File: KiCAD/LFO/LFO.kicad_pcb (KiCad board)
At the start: 2 copper layers, 30 x 100 mm, 16 parts, among them J1 OUT, J2 OUT, J3 Conn_01x03, J4 Conn_01x03, SW1 SW_SPDT, U1 TL072

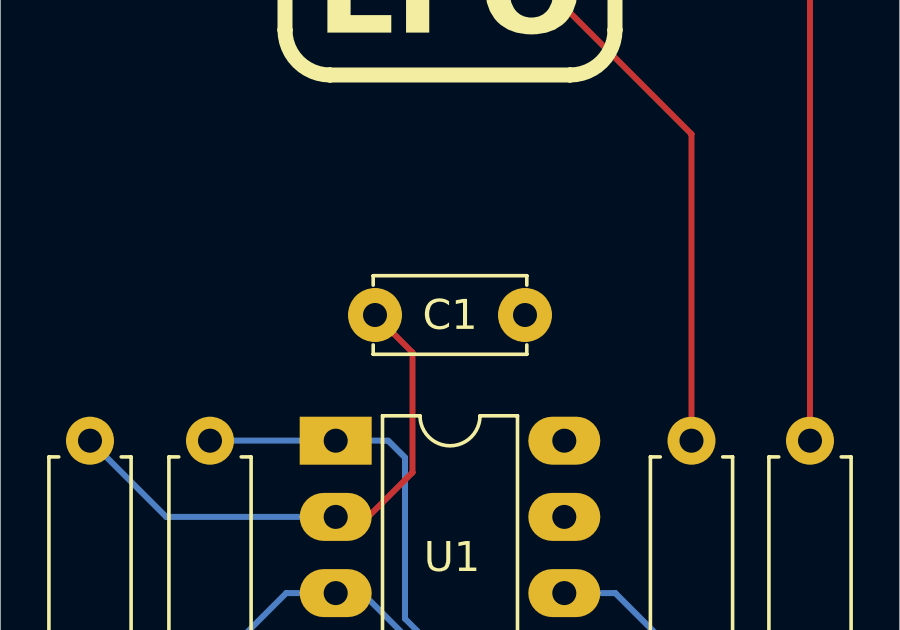
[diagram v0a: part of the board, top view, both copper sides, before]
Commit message: Library updates
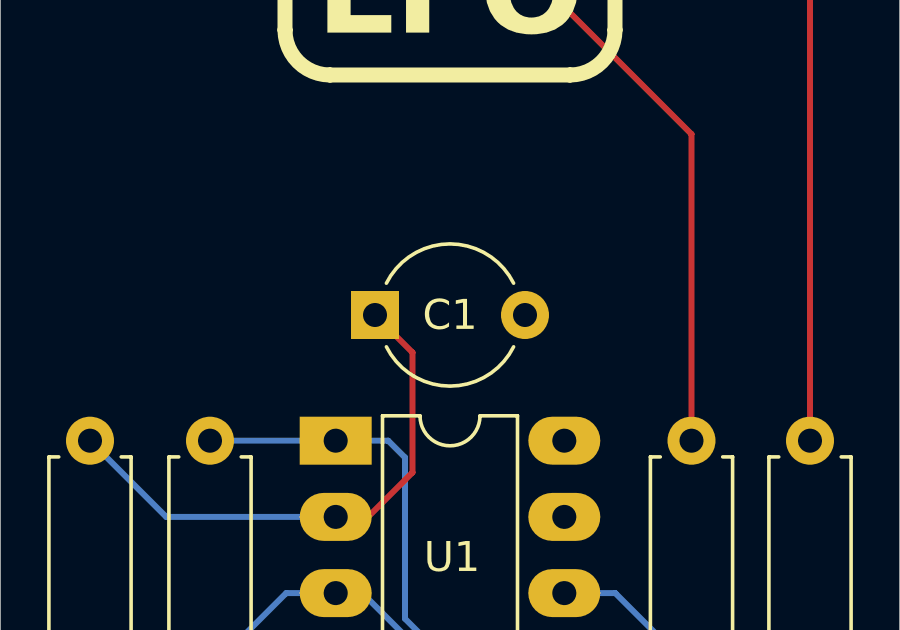
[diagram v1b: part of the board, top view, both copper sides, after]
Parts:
- C1: footprint HackSynth:C_Disc_D5.0mm_W2.5mm_P5.00mm -> HackSynth:C_Radial_Tantal_D4.5mm_P5.00mm
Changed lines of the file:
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@@
 		)
 		(embedded_fonts no)
-		(model "C:/Program Files/KiCad/share/kicad/modules/packages3d/Package_DIP.3dshapes/DIP-8_W7.62mm.step"
+		(model "C:/Users/ocd/OneDrive/Drafting/CCHS/HackSynth/KiCAD/HackSynth.pretty/DIP-8_W7.62mm.step"
 			(offset
 				(xyz -3.81 3.81 0)
@@
 		)
 	)
-	(footprint "HackSynth:C_Disc_D5.0mm_W2.5mm_P5.00mm"
+	(footprint "HackSynth:C_Radial_Tantal_D4.5mm_P5.00mm"
 		(layer "F.Cu")
 		(at 147.5 92)
-		(descr "C, Disc series, Radial, pin pitch=5.00mm, , diameter*width=5*2.5mm^2, Capacitor, http://cdn-reichelt.de/documents/datenblatt/B300/DS_KERKO_TC.pdf")
-		(tags "C Disc series Radial pin pitch 5.00mm  diameter 5mm width 2.5mm Capacitor")
+		(descr "CP, Radial_Tantal series, Radial, pin pitch=5.00mm, diameter=4.5mm, height=10mm, Tantal Electrolytic Capacitor, http://cdn-reichelt.de/documents/datenblatt/B300/TANTAL-TB-Serie%23.pdf")
+		(tags "CP Radial_Tantal series Radial pin pitch 5.00mm diameter 4.5mm height 10mm Tantal Electrolytic Capacitor")
 		(property "Reference" "C1"
 			(at 2.5 0 0)
@@
 		)
 		(property "Value" "2µ2"
-			(at 2.5 -3 0)
+			(at 2.5 3.5 0)
 			(layer "F.Fab")
 			(effects
@@
 		(sheetfile "LFO.kicad_sch")
 		(attr through_hole)
-		(fp_line
-			(start -0.06 -1.31)
-			(end -0.06 -0.996)
+		(fp_arc
+			(start 0.380259 -1.06)
+			(mid 2.5 -2.37)
+			(end 4.619741 -1.06)
 			(stroke
 				(width 0.12)
@@
 			(layer "F.SilkS")
 		)
-		(fp_line
-			(start -0.06 -1.31)
-			(end 5.06 -1.31)
+		(fp_arc
+			(start 4.619741 1.06)
+			(mid 2.5 2.37)
+			(end 0.380259 1.06)
 			(stroke
 				(width 0.12)
@@
 			(layer "F.SilkS")
 		)
-		(fp_line
-			(start -0.06 0.996)
-			(end -0.06 1.31)
-			(stroke
-				(width 0.12)
-				(type solid)
-			)
-			(layer "F.SilkS")
-		)
-		(fp_line
-			(start -0.06 1.31)
-			(end 5.06 1.31)
-			(stroke
-				(width 0.12)
-				(type solid)
-			)
-			(layer "F.SilkS")
-		)
-		(fp_line
-			(start 5.06 -1.31)
-			(end 5.06 -0.996)
-			(stroke
-				(width 0.12)
-				(type solid)
-			)
-			(layer "F.SilkS")
-		)
-		(fp_line
-			(start 5.06 0.996)
-			(end 5.06 1.31)
-			(stroke
-				(width 0.12)
-				(type solid)
-			)
-			(layer "F.SilkS")
-		)
-		(fp_line
-			(start -1.05 -1.6)
-			(end -1.05 1.6)
+		(fp_circle
+			(center 2.5 0)
+			(end 6.22 0)
 			(stroke
 				(width 0.05)
 				(type solid)
 			)
+			(fill no)
 			(layer "F.CrtYd")
 		)
-		(fp_line
-			(start -1.05 1.6)
-			(end 6.05 1.6)
-			(stroke
-				(width 0.05)
-				(type solid)
-			)
-			(layer "F.CrtYd")
-		)
-		(fp_line
-			(start 6.05 -1.6)
-			(end -1.05 -1.6)
-			(stroke
-				(width 0.05)
-				(type solid)
-			)
-			(layer "F.CrtYd")
-		)
-		(fp_line
-			(start 6.05 1.6)
-			(end 6.05 -1.6)
-			(stroke
-				(width 0.05)
-				(type solid)
-			)
-			(layer "F.CrtYd")
-		)
-		(fp_line
-			(start 0 -1.25)
-			(end 0 1.25)
+		(fp_circle
+			(center 2.5 0)
+			(end 4.75 0)
 			(stroke
 				(width 0.1)
 				(type solid)
 			)
-			(layer "F.Fab")
-		)
-		(fp_line
-			(start 0 1.25)
-			(end 5 1.25)
-			(stroke
-				(width 0.1)
-				(type solid)
-			)
-			(layer "F.Fab")
-		)
-		(fp_line
-			(start 5 -1.25)
-			(end 0 -1.25)
-			(stroke
-				(width 0.1)
-				(type solid)
-			)
-			(layer "F.Fab")
-		)
-		(fp_line
-			(start 5 1.25)
-			(end 5 -1.25)
-			(stroke
-				(width 0.1)
-				(type solid)
-			)
+			(fill no)
 			(layer "F.Fab")
 		)
@@
 			(effects
 				(font
-					(size 1 1)
-					(thickness 0.15)
+					(size 0.9 0.9)
+					(thickness 0.135)
 				)
 			)
 		)
-		(pad "1" thru_hole circle
+		(pad "1" thru_hole rect
 			(at 0 0)
-			(size 1.8 1.8)
+			(size 1.6 1.6)
 			(drill 0.8)
 			(layers "*.Cu" "*.Mask")
@@
 		(pad "2" thru_hole circle
 			(at 5 0)
-			(size 1.8 1.8)
+			(size 1.6 1.6)
 			(drill 0.8)
 			(layers "*.Cu" "*.Mask")
@@
 		)
 		(embedded_fonts no)
-		(model "C:/Program Files/KiCad/share/kicad/modules/packages3d/Capacitor_THT.3dshapes/C_Disc_D5.0mm_W2.5mm_P5.00mm.step"
+		(model "${KICAD9_3DMODEL_DIR}/Capacitor_THT.3dshapes/CP_Radial_Tantal_D4.5mm_P5.00mm.wrl"
 			(offset
 				(xyz 0 0 0)

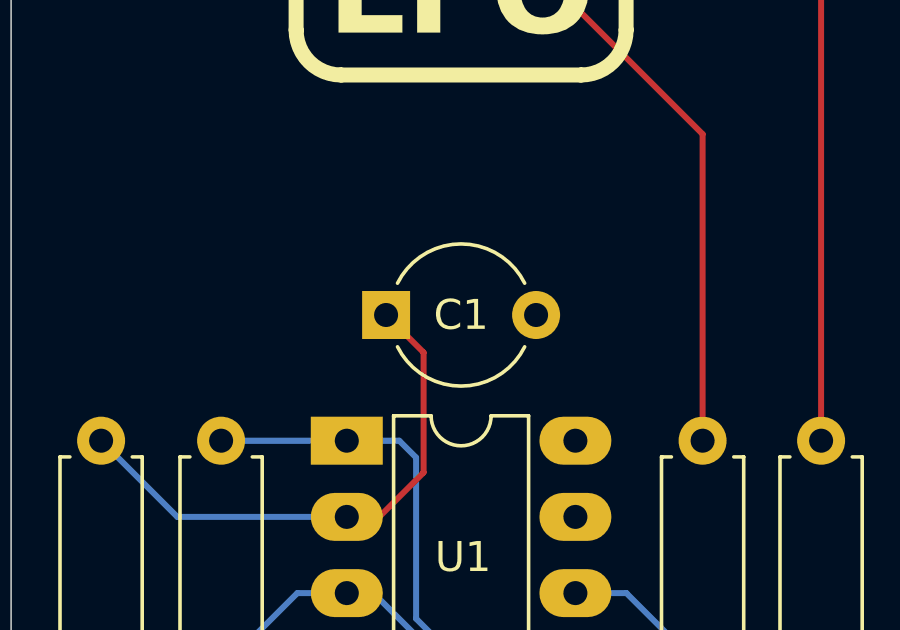
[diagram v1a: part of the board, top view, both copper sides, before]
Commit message: ASDR Schematic + LFO Gerbers
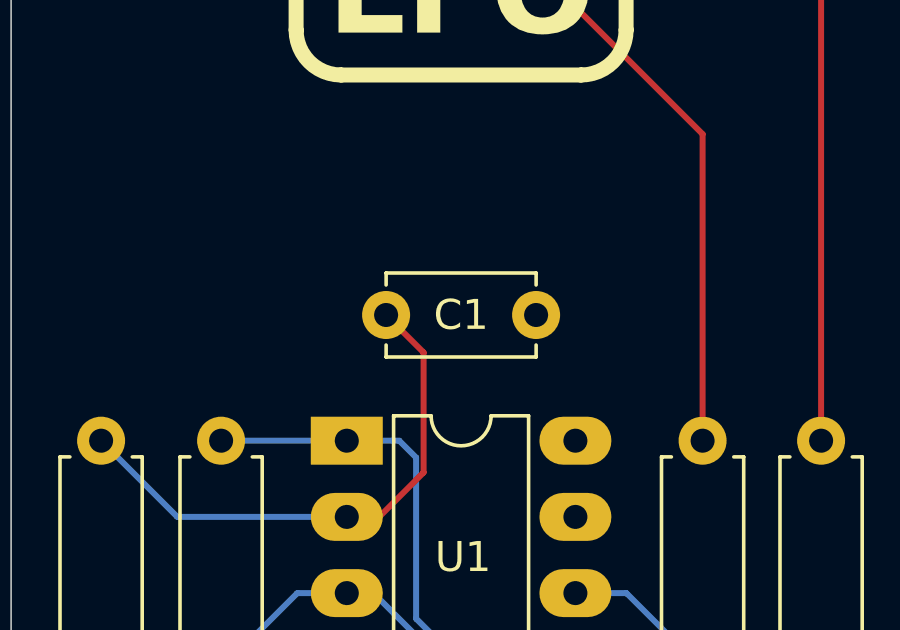
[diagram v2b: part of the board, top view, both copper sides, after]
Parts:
- C1: footprint HackSynth:C_Radial_Tantal_D4.5mm_P5.00mm -> HackSynth:C_Ceramic_D4.5mm_P5.00mm
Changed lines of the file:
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@@
 		(tenting front back)
 		(pcbplotparams
-			(layerselection 0x00000000_00000000_55555555_5755f5ff)
+			(layerselection 0x00000000_00000000_55555555_575555ff)
 			(plot_on_all_layers_selection 0x00000000_00000000_00000000_00000000)
 			(disableapertmacros no)
@@
 			(usegerberattributes yes)
 			(usegerberadvancedattributes yes)
-			(creategerberjobfile yes)
+			(creategerberjobfile no)
 			(dashed_line_dash_ratio 12.000000)
 			(dashed_line_gap_ratio 3.000000)
@@
 			(outputformat 1)
 			(mirror no)
-			(drillshape 1)
+			(drillshape 0)
 			(scaleselection 1)
-			(outputdirectory "")
+			(outputdirectory "Gerbers/")
 		)
 	)
@@
 		)
 	)
-	(footprint "HackSynth:C_Radial_Tantal_D4.5mm_P5.00mm"
+	(footprint "HackSynth:C_Ceramic_D4.5mm_P5.00mm"
 		(layer "F.Cu")
 		(at 147.5 92)
-		(descr "CP, Radial_Tantal series, Radial, pin pitch=5.00mm, diameter=4.5mm, height=10mm, Tantal Electrolytic Capacitor, http://cdn-reichelt.de/documents/datenblatt/B300/TANTAL-TB-Serie%23.pdf")
-		(tags "CP Radial_Tantal series Radial pin pitch 5.00mm diameter 4.5mm height 10mm Tantal Electrolytic Capacitor")
 		(property "Reference" "C1"
-			(at 2.5 0 0)
+			(at 2.5 0.000001 0)
 			(layer "F.SilkS")
 			(effects
@@
 		(sheetfile "LFO.kicad_sch")
 		(attr through_hole)
-		(fp_arc
-			(start 0.380259 -1.06)
-			(mid 2.5 -2.37)
-			(end 4.619741 -1.06)
+		(fp_line
+			(start 0 -1.4)
+			(end 5 -1.4)
 			(stroke
 				(width 0.12)
@@
 			(layer "F.SilkS")
 		)
-		(fp_arc
-			(start 4.619741 1.06)
-			(mid 2.5 2.37)
-			(end 0.380259 1.06)
+		(fp_line
+			(start 0 -1)
+			(end 0 -1.4)
 			(stroke
 				(width 0.12)
@@
 			(layer "F.SilkS")
 		)
-		(fp_circle
-			(center 2.5 0)
-			(end 6.22 0)
+		(fp_line
+			(start 0 1)
+			(end 0 1.4)
 			(stroke
-				(width 0.05)
+				(width 0.12)
 				(type solid)
 			)
+			(layer "F.SilkS")
+		)
+		(fp_line
+			(start 0 1.4)
+			(end 5 1.4)
+			(stroke
+				(width 0.12)
+				(type solid)
+			)
+			(layer "F.SilkS")
+		)
+		(fp_line
+			(start 5 -1.4)
+			(end 5 -1)
+			(stroke
+				(width 0.12)
+				(type solid)
+			)
+			(layer "F.SilkS")
+		)
+		(fp_line
+			(start 5 1.4)
+			(end 5 1)
+			(stroke
+				(width 0.12)
+				(type solid)
+			)
+			(layer "F.SilkS")
+		)
+		(fp_rect
+			(start -0.8 -1.5)
+			(end 5.8 1.5)
+			(stroke
+				(width 0.05)
+				(type default)
+			)
 			(fill no)
 			(layer "F.CrtYd")
 		)
-		(fp_circle
-			(center 2.5 0)
-			(end 4.75 0)
+		(fp_line
+			(start 0.1 -1.3)
+			(end 4.9 -1.3)
 			(stroke
 				(width 0.1)
-				(type solid)
+				(type default)
+			)
+			(layer "F.Fab")
+		)
+		(fp_line
+			(start 0.1 -0.9)
+			(end 0.1 -1.3)
+			(stroke
+				(width 0.1)
+				(type default)
+			)
+			(layer "F.Fab")
+		)
+		(fp_line
+			(start 0.1 0.9)
+			(end 0.1 1.3)
+			(stroke
+				(width 0.1)
+				(type default)
+			)
+			(layer "F.Fab")
+		)
+		(fp_line
+			(start 0.1 1.3)
+			(end 4.9 1.3)
+			(stroke
+				(width 0.1)
+				(type default)
+			)
+			(layer "F.Fab")
+		)
+		(fp_line
+			(start 4.9 -1.3)
+			(end 4.9 -0.9)
+			(stroke
+				(width 0.1)
+				(type default)
+			)
+			(layer "F.Fab")
+		)
+		(fp_line
+			(start 4.9 0.9)
+			(end 4.9 1.3)
+			(stroke
+				(width 0.1)
+				(type default)
 			)
-			(fill no)
 			(layer "F.Fab")
 		)
@@
 			)
 		)
-		(pad "1" thru_hole rect
+		(pad "1" thru_hole circle
 			(at 0 0)
 			(size 1.6 1.6)
@@
 		)
 		(embedded_fonts no)
-		(model "${KICAD9_3DMODEL_DIR}/Capacitor_THT.3dshapes/CP_Radial_Tantal_D4.5mm_P5.00mm.wrl"
+		(model "C:/Users/ocd/OneDrive/Drafting/CCHS/HackSynth/KiCAD/HackSynth.pretty/C_Ceramic_D4.5mm_P5.00mm.step"
 			(offset
 				(xyz 0 0 0)
@@
 		(stroke
 			(width 0.3)
-			(type default)
+			(type solid)
 		)
 		(layer "F.SilkS")
@@
 		(stroke
 			(width 0.3)
-			(type default)
+			(type solid)
 		)
 		(layer "F.SilkS")
